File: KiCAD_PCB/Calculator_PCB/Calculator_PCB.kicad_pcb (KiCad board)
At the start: 2 copper layers, 109 parts, among them J1 USB_B_Micro, SW1 SW_SPST, SW10 SW_SPST, SW11 SW_SPST, SW12 SW_SPST, SW13 SW_SPST, SW14 SW_SPST, SW15 SW_SPST, SW16 SW_SPST, SW17 SW_SPST, SW18 SW_SPST, SW19 SW_SPST, SW2 SW_SPST, SW20 SW_SPST, SW21 SW_SPST, SW22 SW_SPST, SW23 SW_SPST, SW24 SW_SPST, SW25 SW_SPST, SW26 SW_SPST, SW27 SW_SPST, SW28 SW_SPST, SW29 SW_SPST, SW3 SW_SPST, SW30 SW_SPST, SW31 SW_SPST, SW32 SW_SPST, SW33 SW_SPST, SW34 SW_SPST, SW35 SW_SPST, SW36 SW_SPST, SW37 SW_SPST, SW38 SW_SPST, SW39 SW_SPST, SW4 SW_SPST, SW40 SW_SPST, SW5 SW_SPST, SW6 SW_SPST, SW7 SW_SPST, SW8 SW_SPST, SW9 SW_SPST, U1 W25Q128JVS, U2 RP2040, U3 NCP1117-3.3_SOT223, X1 JTAG-CORTEX, Y1 ABLS-12.000MHZ-B4-T

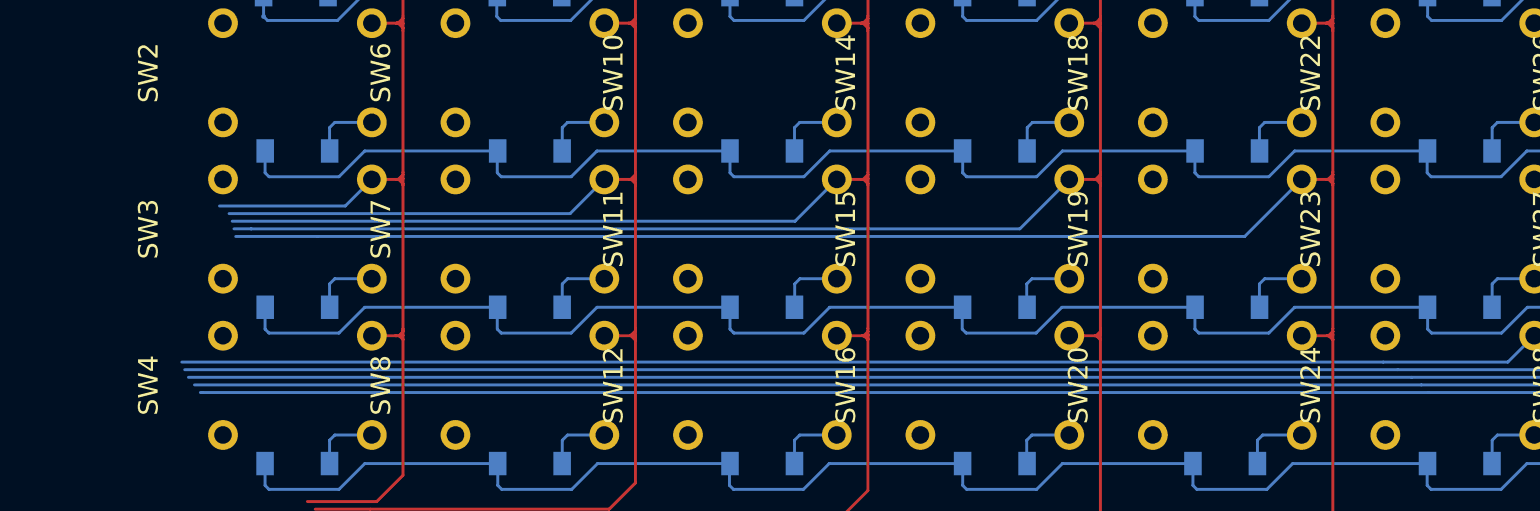
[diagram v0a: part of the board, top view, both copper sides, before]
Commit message: PCB Updates
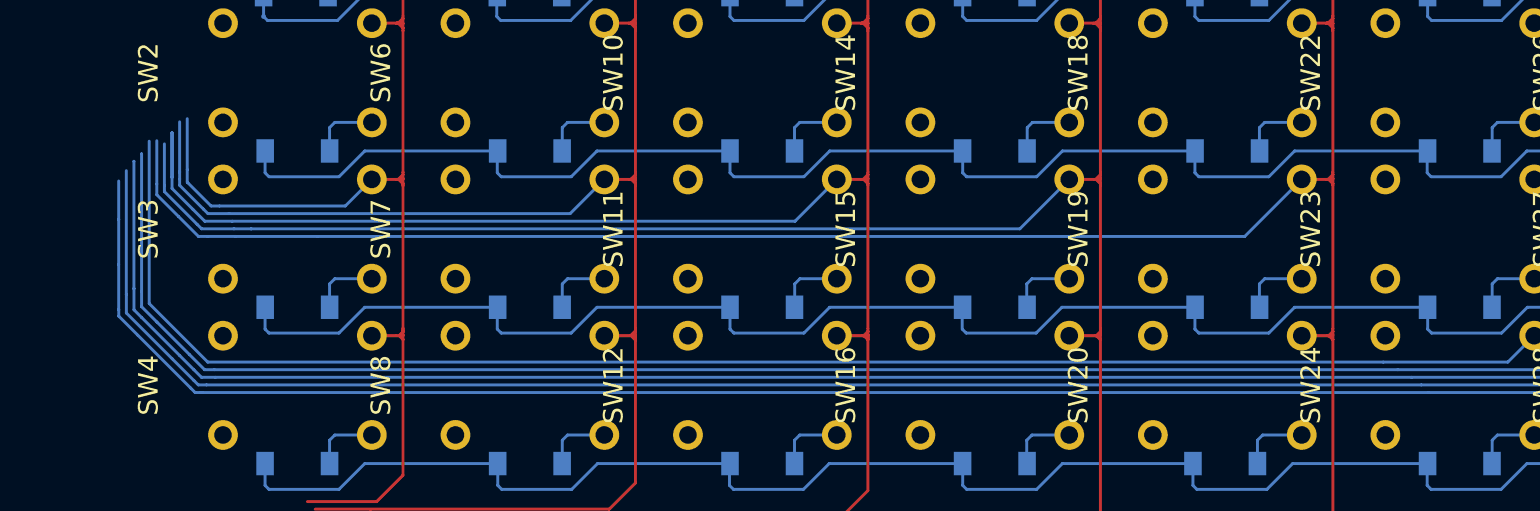
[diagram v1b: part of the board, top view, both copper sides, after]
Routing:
- net /Col12: track 159.6 -> 172.3 mm
- net /Col11: track 147.8 -> 160.1 mm
- net /Col10: track 139.5 -> 151.3 mm
- net /Col9: track 127.9 -> 139.2 mm
- net /Col8: track 116.3 -> 127.5 mm
- net /Col5: track 95.6 -> 104.6 mm
- net /Col7: track 102.2 -> 109.9 mm
- net /Col6: track 91.0 -> 97.8 mm
- net /Col4: track 82.8 -> 89.2 mm
- net /Col3: track 59.1 -> 64.5 mm
